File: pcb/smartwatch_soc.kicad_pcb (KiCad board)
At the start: 2 copper layers, 31 parts, among them J2 USB_B_Micro, SW1 CK_KMS2xxGP, SW2 Button, SW3 Button, SW4 Button, SW5 Button, SW7 CK_KMS2xxGP, U1 MIC5219-3.3YM5, U2 LSM6DS3, U3 OLED_Display, U5 ESP32-S3-MINI-1

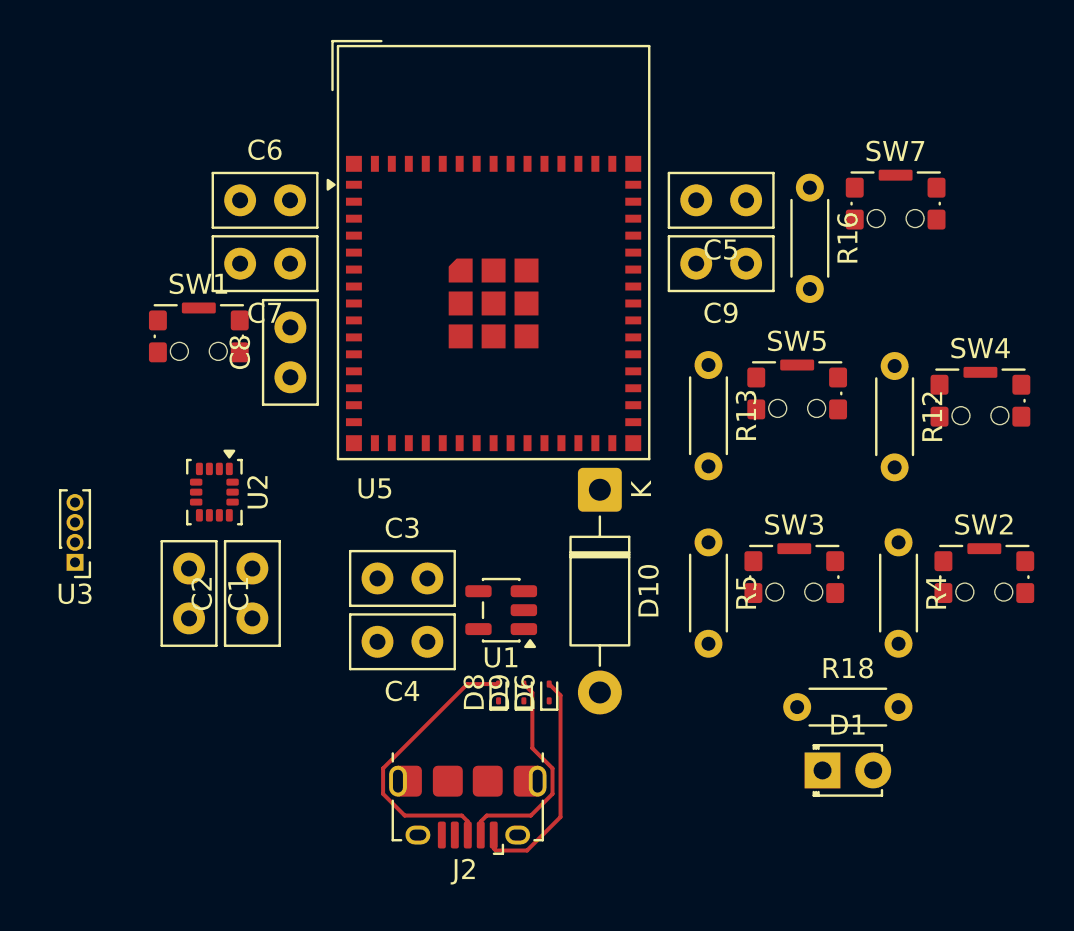
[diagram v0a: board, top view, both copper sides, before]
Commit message: pcb design
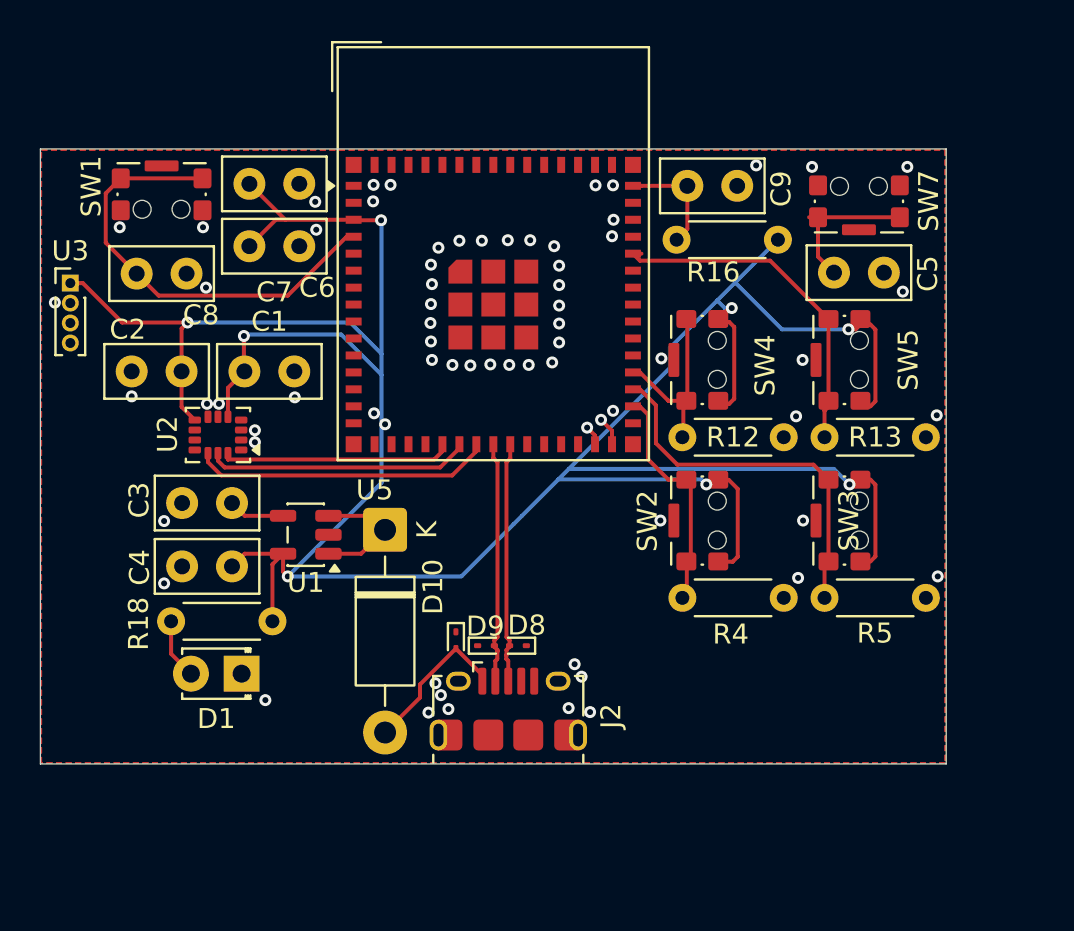
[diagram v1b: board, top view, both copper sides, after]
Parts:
- moved D1 29.5 mm to (148.7, 87.2), turned to 180 degrees
- moved R18 26.6 mm to (150.2, 84.6), turned to 180 degrees
- moved SW2 14.4 mm to (171.8, 79.5), turned to 90 degrees
- moved SW4 14.1 mm to (171.8, 71.5), turned to 90 degrees
- moved U3 14.0 mm to (140.1, 67.7), turned to 0 degrees
- moved C2 13.8 mm to (143.2, 72.1), turned to 0 degrees
- moved R12 11.2 mm to (170.8, 75.4), turned to 0 degrees
- moved R4 11.2 mm to (170.8, 83.4), turned to 0 degrees
- moved D10 11.0 mm to (155.9, 80.0)
- moved C3 10.5 mm to (145.7, 78.7)
- moved C4 10.5 mm to (148.2, 81.8)
- moved U1 10.5 mm to (151.9, 80.3)
- moved C1 10.3 mm to (148.8, 72.1), turned to 0 degrees
- moved C5 7.80 mm to (180.9, 67.1)
- moved SW1 7.36 mm to (144.7, 63.2)
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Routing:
- net VCC_3V3: track 0.00 -> 157.4 mm, vias 0 -> 8
- net ESP32_GPIO48: track 0.00 -> 30.8 mm, vias 0 -> 1
- net ESP32_GPIO34: track 0.00 -> 30.4 mm, vias 0 -> 1
- net ESP32_GPIO0: track 0.00 -> 22.4 mm
- net ESP32_GPIO37: track 0.00 -> 18.8 mm
- net ESP32_GPIO45: track 0.00 -> 17.9 mm
- net ESP32_GPIO18: track 0.00 -> 15.0 mm
- net ESP32_EN: track 0.00 -> 13.7 mm
- net ESP32_GPIO17: track 0.00 -> 13.2 mm
- net ESP32_GPIO16: track 0.00 -> 11.6 mm
- net ESP32_GPIO36: track 0.00 -> 11.5 mm
- net ESP32_GPIO38: track 0.00 -> 9.27 mm
- net VCC_5V: track 0.00 -> 6.46 mm
- net Net-(D1-A): track 0.00 -> 3.04 mm
- net VBUS: track 11.7 -> 8.74 mm
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- added copper zone on B.Cu, net GND
- added copper zone on F.Cu, net GND
- added copper zone on In1.Cu, net GND
- added copper zone on In2.Cu, net GND
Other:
- board outline added: 45.4 x 30.8 mm
- copper layers 2 -> 4
